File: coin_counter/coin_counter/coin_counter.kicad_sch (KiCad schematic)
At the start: 13 parts, among them J1 Q_EMT, J2 N_EMT, J3 P_EMT, J4 D_EMT, J5 Mom, J6 D_RCV, J7 P_RCV, J8 N_RCV, J9 Q_RCV

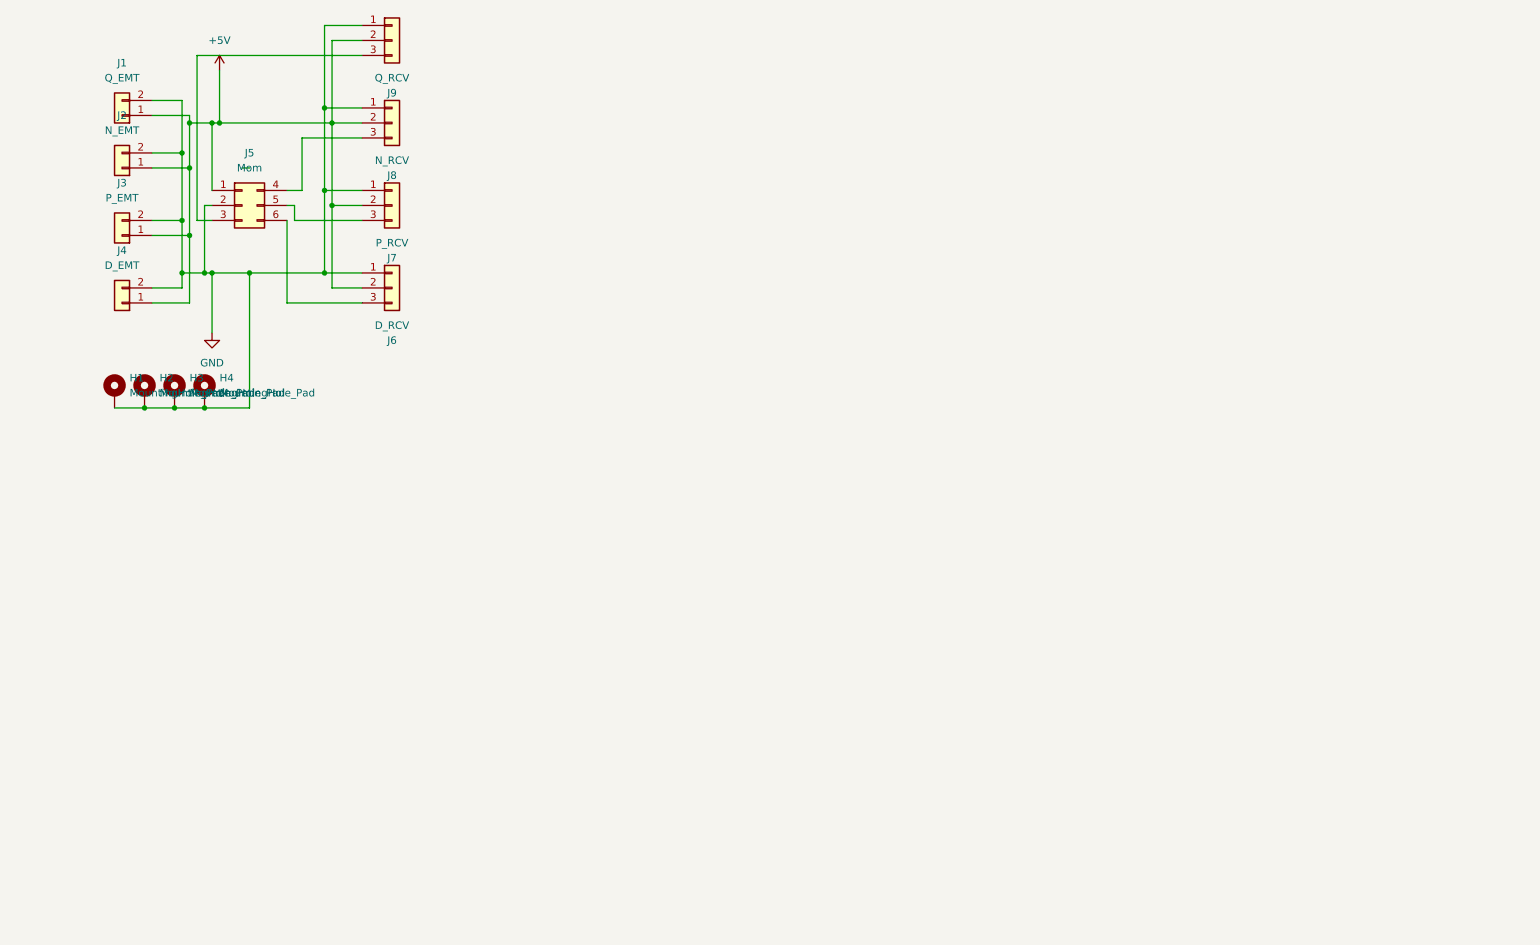
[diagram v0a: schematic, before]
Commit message: more
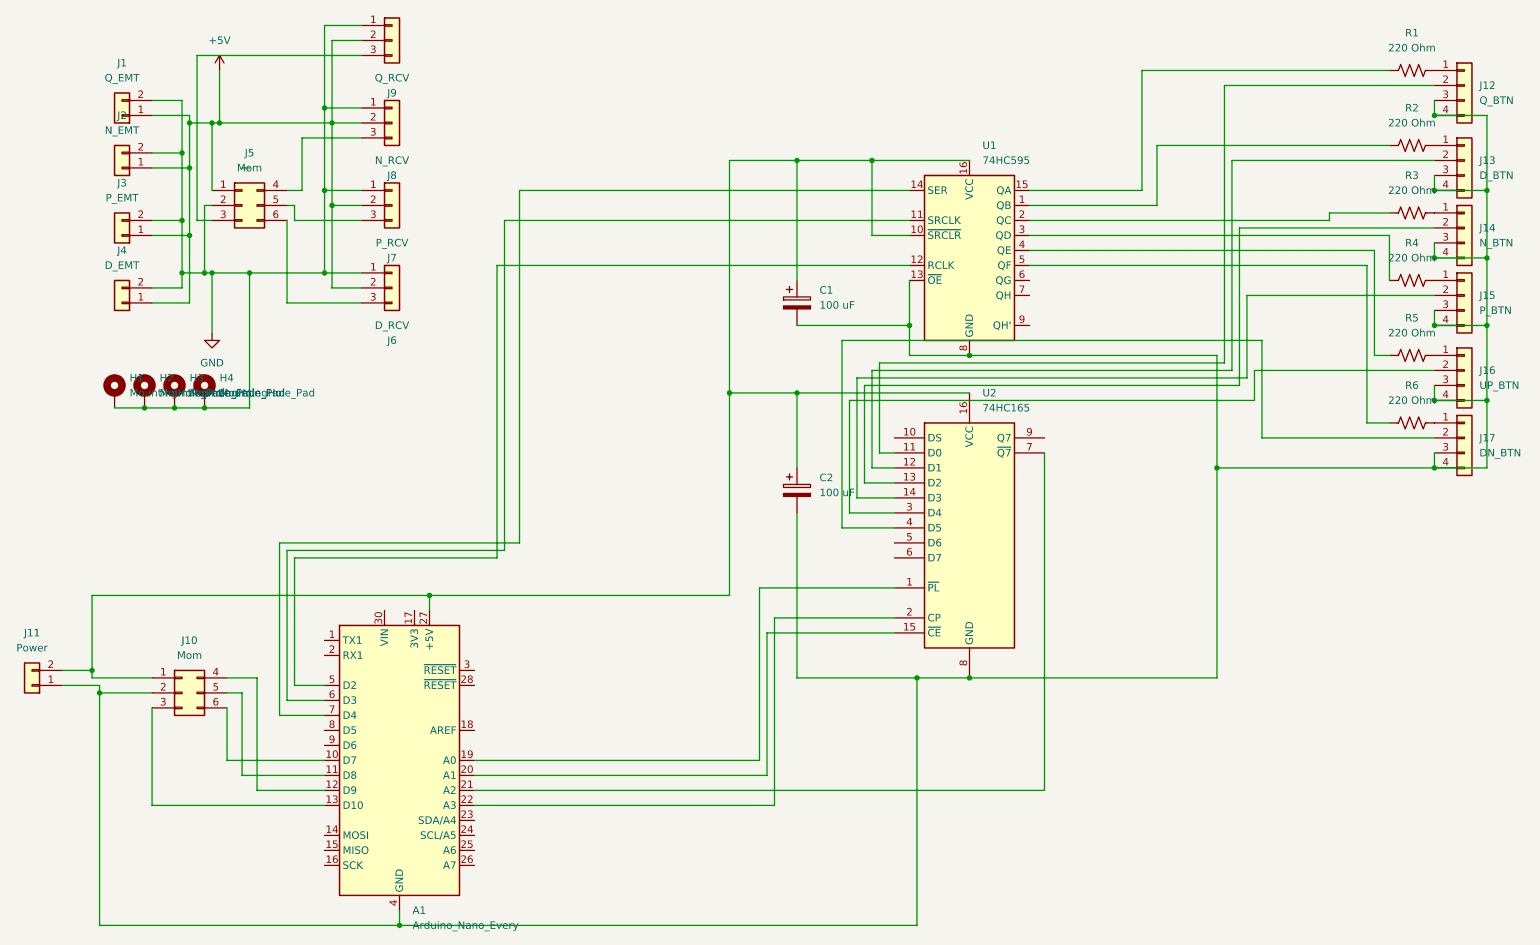
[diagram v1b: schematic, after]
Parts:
- added A1: Arduino_Nano_Every, Module:Arduino_Nano, symbol MCU_Module:Arduino_Nano_Every
- added C1, C2: 100 uF, symbol Device:C_Polarized
- added J10: Mom, Connector_JST:JST_XH_B6B-XH-A_1x06_P2.50mm_Vertical, symbol Connector_Generic:Conn_02x03_Top_Bottom
- added J11: Power, Connector_JST:JST_XH_B2B-XH-A_1x02_P2.50mm_Vertical, symbol Connector_Generic:Conn_01x02
- added J12: Q_BTN, symbol Connector_Generic:Conn_01x04
- added J13: D_BTN, symbol Connector_Generic:Conn_01x04
- added J14: N_BTN, symbol Connector_Generic:Conn_01x04
- added J15: P_BTN, symbol Connector_Generic:Conn_01x04
- added J16: UP_BTN, symbol Connector_Generic:Conn_01x04
- added J17: DN_BTN, symbol Connector_Generic:Conn_01x04
- added R1, R2, R3, R4, R5, R6: 220 Ohm, Resistor_THT:R_Axial_DIN0204_L3.6mm_D1.6mm_P5.08mm_Vertical, symbol Device:R_US
- added U1: 74HC595, Package_SO:SO-16_3.9x9.9mm_P1.27mm, symbol 74xx:74HC595
- added U2: 74HC165, Package_SO:SO-16_3.9x9.9mm_P1.27mm, symbol 74xx:74HC165
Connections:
- new net: J15.1 (Pin_1), R4.2
- new net: J15.2 (Pin_2), U2.14 (D3)
- new net: A1.29 (GND), A1.4 (GND), C1.2, C2.2, J10.2 (Pin_2), J11.1 (Pin_1), J12.3 (Pin_3), J12.4 (Pin_4), J13.3 (Pin_3), J13.4 (Pin_4), J14.3 (Pin_3), J14.4 (Pin_4), J15.3 (Pin_3), J15.4 (Pin_4), J16.3 (Pin_3), J16.4 (Pin_4), J17.3 (Pin_3), J17.4 (Pin_4), U1.13 (~{OE}), U1.8 (GND), U2.8 (GND)
- new net: A1.19 (A0), U2.1 (~{PL})
- new net: J12.2 (Pin_2), U2.11 (D0)
- new net: J13.2 (Pin_2), U2.12 (D1)
- new net: J14.2 (Pin_2), U2.13 (D2)
- new net: A1.20 (A1), U2.15 (~{CE})
- new net: A1.27 (+5V), C1.1, C2.1, J10.1 (Pin_1), J11.2 (Pin_2), U1.10 (~{SRCLR}), U1.16 (VCC), U2.16 (VCC)
- new net: A1.22 (A3), U2.2 (CP)
- new net: J16.2 (Pin_2), U2.3 (D4)
- new net: J17.2 (Pin_2), U2.4 (D5)
- new net: A1.21 (A2), U2.7 (~{Q7})
- new net: R2.1, U1.1 (QB)
- new net: A1.6 (D3), U1.11 (SRCLK)
- new net: A1.5 (D2), U1.12 (RCLK)
- new net: A1.7 (D4), U1.14 (SER)
- new net: R1.1, U1.15 (QA)
- new net: R3.1, U1.2 (QC)
- new net: R4.1, U1.3 (QD)
- new net: R5.1, U1.4 (QE)
- new net: R6.1, U1.5 (QF)
- new net: J17.1 (Pin_1), R6.2
- new net: J14.1 (Pin_1), R3.2
- new net: J16.1 (Pin_1), R5.2
- new net: A1.10 (D7), J10.6 (Pin_6)
- new net: A1.11 (D8), J10.5 (Pin_5)
- new net: A1.12 (D9), J10.4 (Pin_4)
- new net: A1.13 (D10), J10.3 (Pin_3)
- new net: J13.1 (Pin_1), R2.2
- new net: J12.1 (Pin_1), R1.2
